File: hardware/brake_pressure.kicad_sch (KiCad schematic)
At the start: 13 parts, among them U6 MCP6002-xMC

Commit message: Add 0R resistors to the brake pressure signals
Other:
- company: (none) -> S. Sambor
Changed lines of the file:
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@@
 (kicad_sch (version 20230121) (generator eeschema)
   (paper "A4")
+  (title_block
+    (rev "2.0")
+    (company "S. Sambor")
+    (comment 1 "J. Jurczak")
+    (comment 2 "P. Gawron")
+    (comment 3 "I. Kajdan")
+  )
   (junction (at 200.66 90.17) (diameter 0) (color 0 0 0 0)
   )

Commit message: Change test points footprints
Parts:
- TP7: value ~ -> BR_P; footprint TestPoint:TestPoint_Pad_1.0x1.0mm -> TestPoint:TestPoint_Pad_D1.0mm
- TP7: value OUT -> BR_OUT; footprint TestPoint:TestPoint_Pad_1.0x1.0mm -> TestPoint:TestPoint_Pad_D1.0mm
- TP7: value ~ -> BR_MID; footprint TestPoint:TestPoint_Pad_1.0x1.0mm -> TestPoint:TestPoint_Pad_D1.0mm
- TP7: value ~ -> BR_N; footprint TestPoint:TestPoint_Pad_1.0x1.0mm -> TestPoint:TestPoint_Pad_D1.0mm
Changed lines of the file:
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@@
       (effects (font (size 1.27 1.27)) (justify left))
     )
-    (property "Value" "~" (at 119.38 90.043 0)
+    (property "Value" "BR_P" (at 119.38 90.043 0)
       (effects (font (size 1.27 1.27)) (justify left) hide)
     )
-    (property "Footprint" "TestPoint:TestPoint_Pad_1.0x1.0mm" (at 121.92 91.44 0)
+    (property "Footprint" "TestPoint:TestPoint_Pad_D1.0mm" (at 121.92 91.44 0)
       (effects (font (size 1.27 1.27)) hide)
     )
@@
       (effects (font (size 1.27 1.27)) (justify left))
     )
-    (property "Value" "OUT" (at 175.26 95.123 0)
+    (property "Value" "BR_OUT" (at 175.26 95.123 0)
       (effects (font (size 1.27 1.27)) (justify left) hide)
     )
-    (property "Footprint" "TestPoint:TestPoint_Pad_1.0x1.0mm" (at 177.8 96.52 0)
+    (property "Footprint" "TestPoint:TestPoint_Pad_D1.0mm" (at 177.8 96.52 0)
       (effects (font (size 1.27 1.27)) hide)
     )
@@
       (effects (font (size 1.27 1.27)) (justify left))
     )
-    (property "Value" "~" (at 148.59 92.583 0)
+    (property "Value" "BR_MID" (at 148.59 92.583 0)
       (effects (font (size 1.27 1.27)) (justify left) hide)
     )
-    (property "Footprint" "TestPoint:TestPoint_Pad_1.0x1.0mm" (at 151.13 93.98 0)
+    (property "Footprint" "TestPoint:TestPoint_Pad_D1.0mm" (at 151.13 93.98 0)
       (effects (font (size 1.27 1.27)) hide)
     )
@@
       (effects (font (size 1.27 1.27)) (justify left))
     )
-    (property "Value" "~" (at 114.3 97.917 0)
+    (property "Value" "BR_N" (at 114.3 97.917 0)
       (effects (font (size 1.27 1.27)) (justify left) hide)
     )
-    (property "Footprint" "TestPoint:TestPoint_Pad_1.0x1.0mm" (at 111.76 96.52 0)
-      (effects (font (size 1.27 1.27)) hide)
-    )
+    (property "Footprint" "TestPoint:TestPoint_Pad_D1.0mm" (at 111.76 96.52 0)
+      (effects (font (size 1.27 1.27)) hide)
+    )

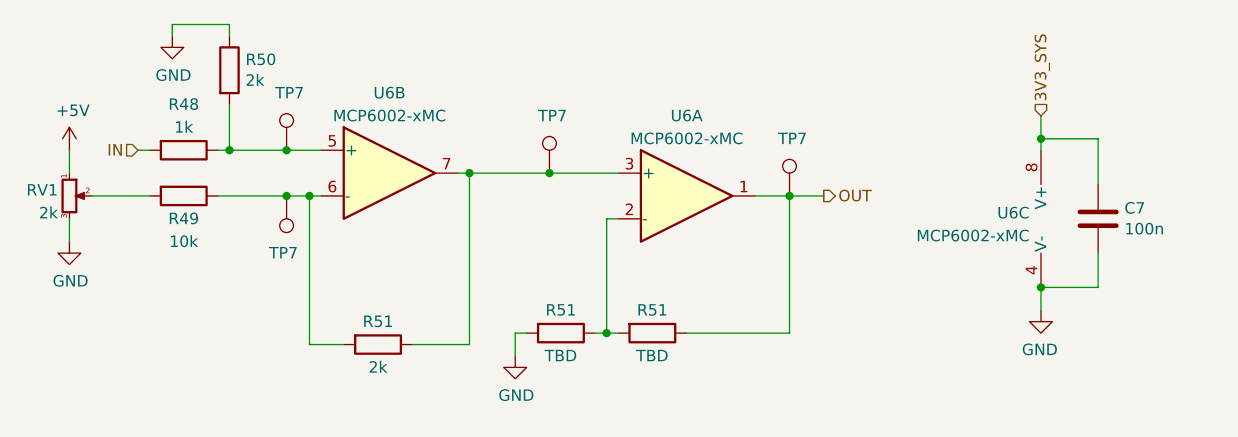
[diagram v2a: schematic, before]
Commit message: Refactor
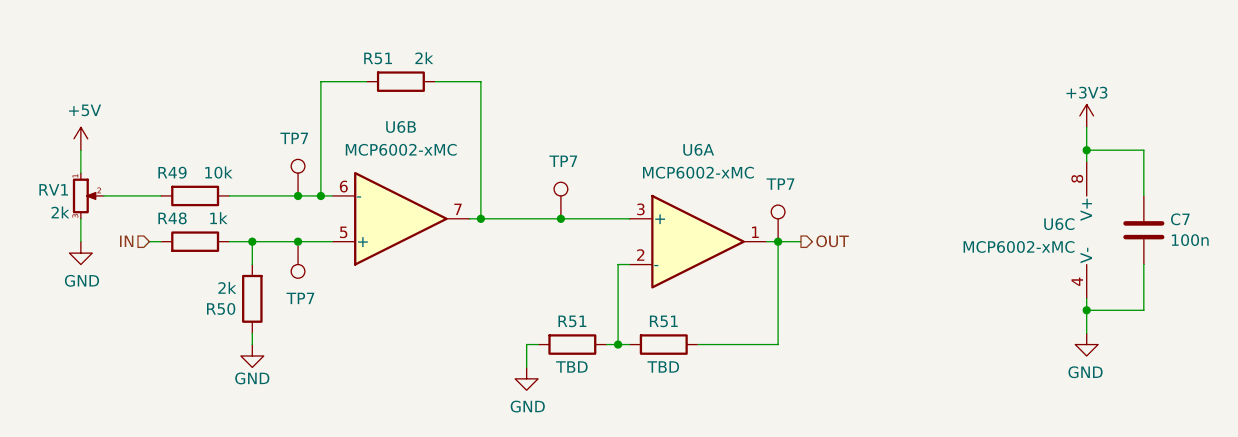
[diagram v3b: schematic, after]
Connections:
- net 3V3_SYS renamed +3V3
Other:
- moved on the sheet: C7, R48, R49, R50, R51, RV1, TP7, U6A, U6B, U6C
